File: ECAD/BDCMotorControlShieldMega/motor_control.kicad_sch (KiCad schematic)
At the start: 4 parts, among them U23 MCP6S26

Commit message: Progressed ECAD.
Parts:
- U23: Status (none) -> OK
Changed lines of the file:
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@@
+			)
+		)
+		(property "Status" "OK"
+			(at 116.84 95.25 0)
+			(effects
+				(font
+					(size 1.27 1.27)
+				)
+				(hide yes)
 			)
 		)

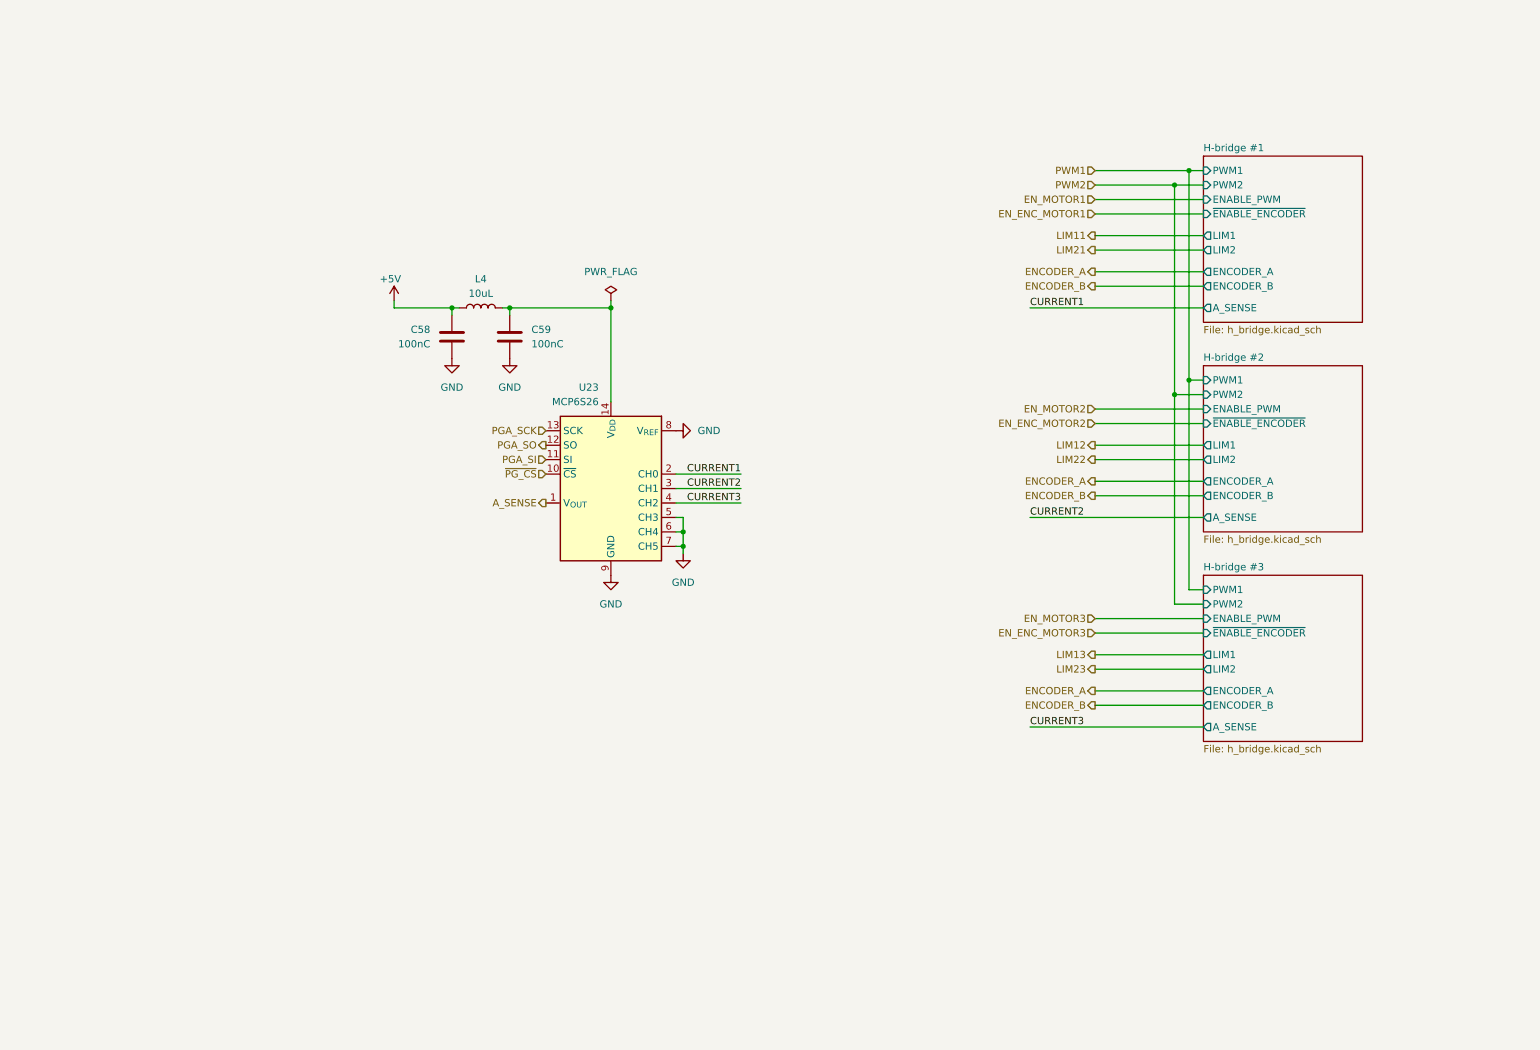
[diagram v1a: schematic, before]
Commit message: Progressed ECAD.
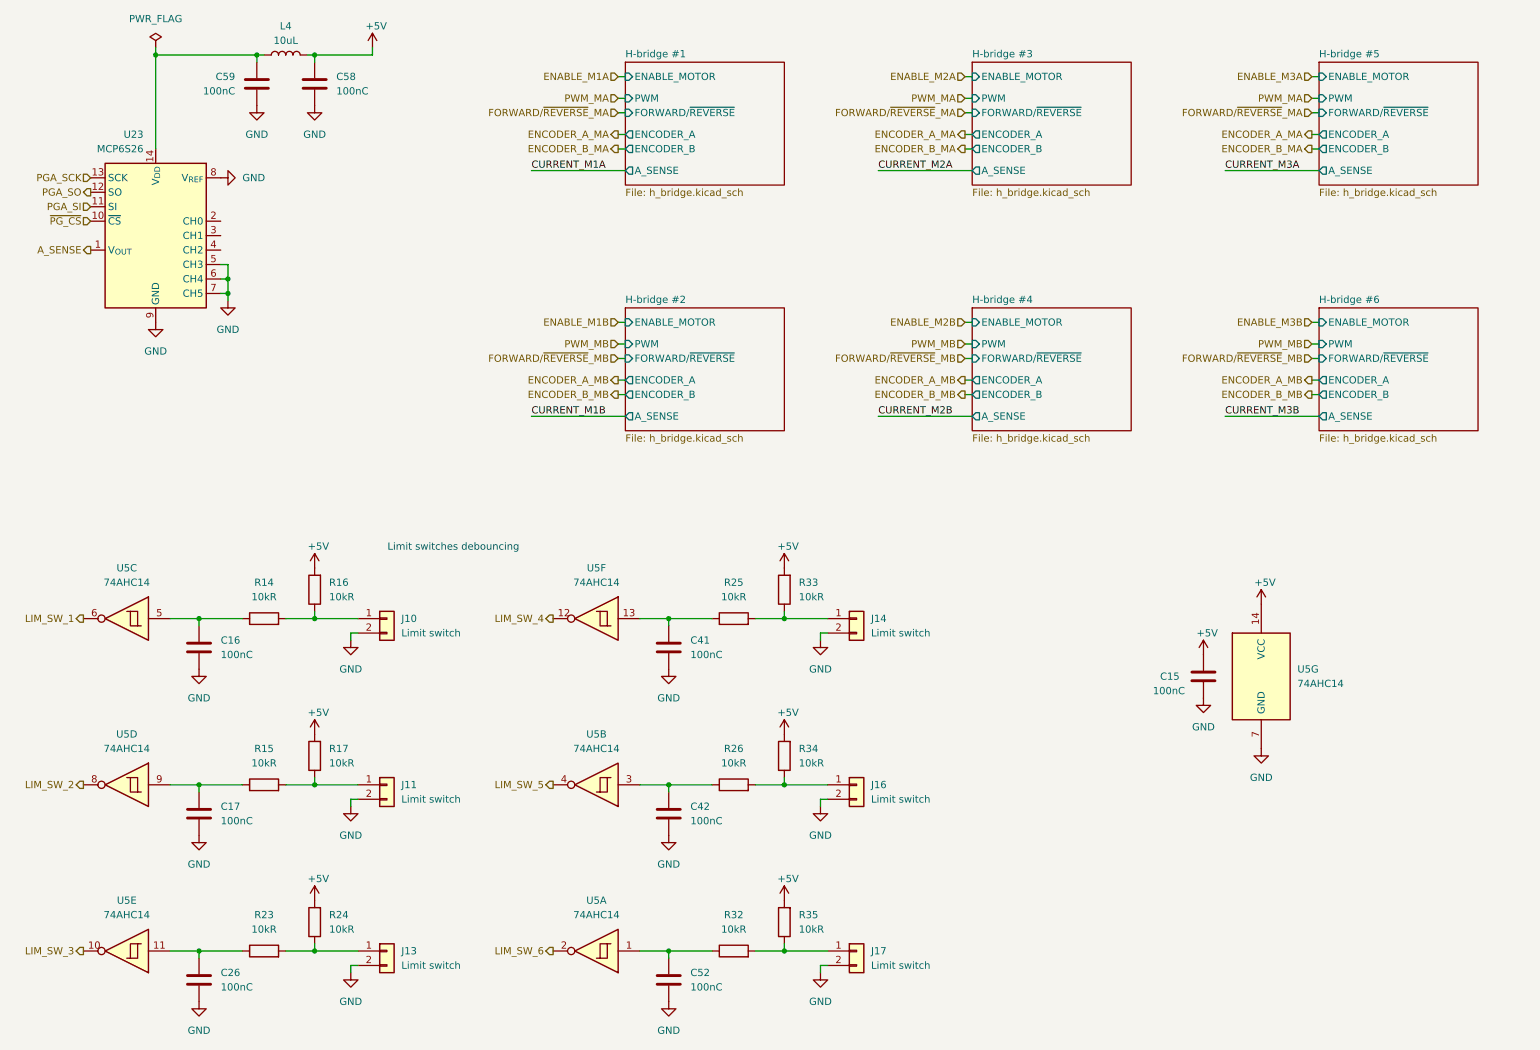
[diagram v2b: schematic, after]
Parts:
- added C15, C16, C17, C26, C41, C42, C52: 100nC, Capacitor_SMD:C_0805_2012Metric, symbol Device:C
- added J10, J11, J13, J14, J16, J17: Limit switch, Connector_JST:JST_PH_B2B-PH-K_1x02_P2.00mm_Vertical, symbol Connector_Generic:Conn_01x02
- added R14, R15, R16, R17, R23, R24, R25, R26, R32, R33, R34, R35: 10kR, Resistor_SMD:R_0805_2012Metric, symbol Device:R
- added U5: 74AHC14, Package_SO:TSSOP-14_4.4x5mm_P0.65mm, symbol 74xx:74HC14
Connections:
- net +5V: now also C15.1, R16.2, R17.2, R24.2, R33.2, R34.2, R35.2, U5.14 (VCC)
- net GND: now also C15.2, C16.2, C17.2, C26.2, C41.2, C42.2, C52.2, J10.2 (Pin_2), J11.2 (Pin_2), J13.2 (Pin_2), J14.2 (Pin_2), J16.2 (Pin_2), J17.2 (Pin_2), U5.7 (GND)
- net CURRENT1: no longer names the net of U23.2 (CH0)
- net CURRENT2: no longer names the net of U23.3 (CH1)
- net CURRENT3: no longer names the net of U23.4 (CH2)
- new net: J16.1 (Pin_1), R26.2, R34.1
- new net: J17.1 (Pin_1), R32.2, R35.1
- new net: C16.1, R14.1, U5.5
- new net: J13.1 (Pin_1), R23.2, R24.1
- new net: J14.1 (Pin_1), R25.2, R33.1
- new net: C41.1, R25.1, U5.13
- new net: C17.1, R15.1, U5.9
- new net: J11.1 (Pin_1), R15.2, R17.1
- new net: C26.1, R23.1, U5.11
- new net: J10.1 (Pin_1), R14.2, R16.1
- new net: C52.1, R32.1, U5.1
- new net: C42.1, R26.1, U5.3
- new net LIM_SW_1: U5.6
- new net LIM_SW_2: U5.8
- new net LIM_SW_3: U5.10
- new net LIM_SW_4: U5.12
- new net LIM_SW_5: U5.4
- new net LIM_SW_6: U5.2
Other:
- added sheet H-bridge #4 (h_bridge.kicad_sch)
- added sheet H-bridge #5 (h_bridge.kicad_sch)
- added sheet H-bridge #6 (h_bridge.kicad_sch)
- sheet H-bridge #1 ports: added ENABLE_MOTOR, FORWARD/~{REVERSE}, PWM; removed ENABLE_PWM, LIM1, LIM2, PWM1, PWM2, ~{ENABLE_ENCODER}
- sheet H-bridge #2 ports: added ENABLE_MOTOR, FORWARD/~{REVERSE}, PWM; removed ENABLE_PWM, LIM1, LIM2, PWM1, PWM2, ~{ENABLE_ENCODER}
- sheet H-bridge #3 ports: added ENABLE_MOTOR, FORWARD/~{REVERSE}, PWM; removed ENABLE_PWM, LIM1, LIM2, PWM1, PWM2, ~{ENABLE_ENCODER}
- note added: "Limit switches debouncing"
- moved on the sheet: C58, C59, L4, U23

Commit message: Progressed ECAD.
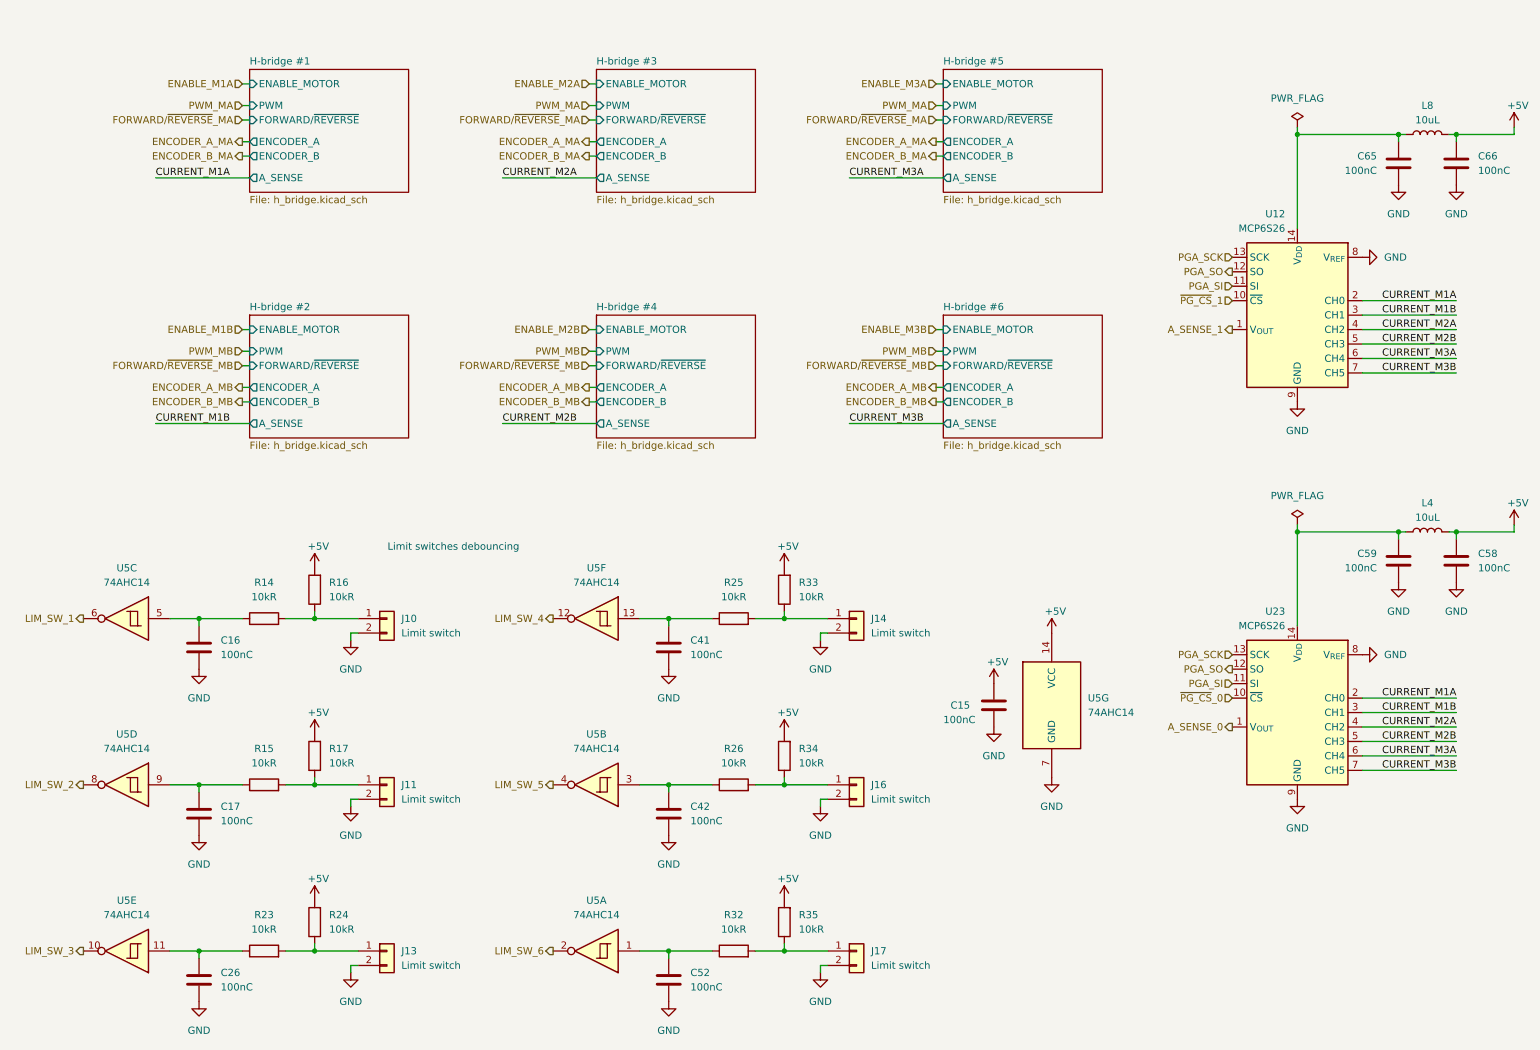
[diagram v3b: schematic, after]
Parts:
- added C65, C66: 100nC, Capacitor_SMD:C_0805_2012Metric, symbol Device:C
- added L8: 10uL, Inductor_SMD:L_0805_2012Metric, symbol Device:L
- added U12: MCP6S26, Package_SO:SOIC-14_3.9x8.7mm_P1.27mm, symbol Analog_custom:MCP6S26
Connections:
- net +5V: now also C66.1, L8.1
- net CURRENT_M1A: now also U23.2 (CH0), U12.2 (CH0)
- net CURRENT_M1B: now also U23.3 (CH1), U12.3 (CH1)
- net CURRENT_M2A: now also U23.4 (CH2), U12.4 (CH2)
- net CURRENT_M2B: now also U23.5 (CH3), U12.5 (CH3)
- net CURRENT_M3A: now also U23.6 (CH4), U12.6 (CH4)
- net CURRENT_M3B: now also U23.7 (CH5), U12.7 (CH5)
- net GND: now also C65.2, C66.2, U12.8 (V_{REF}), U12.9 (GND); no longer U23.5 (CH3), U23.6 (CH4), U23.7 (CH5)
- net PGA_SCK: now also U12.13 (SCK)
- net PGA_SI: now also U12.11 (SI)
- net PGA_SO: now also U12.12 (SO)
- net A_SENSE renamed A_SENSE_0
- net ~{PG_CS} renamed ~{PG_CS}_0
- new net: C65.1, L8.2, U12.14 (V_{DD})
- new net A_SENSE_1: U12.1 (V_{OUT})
- new net ~{PG_CS}_1: U12.10 (~{CS})
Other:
- moved on the sheet: C15, C58, C59, L4, U23, U5G
